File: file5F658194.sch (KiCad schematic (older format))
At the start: 21 parts, among them Q10 SUD50P10-43L, Q11 TIP120

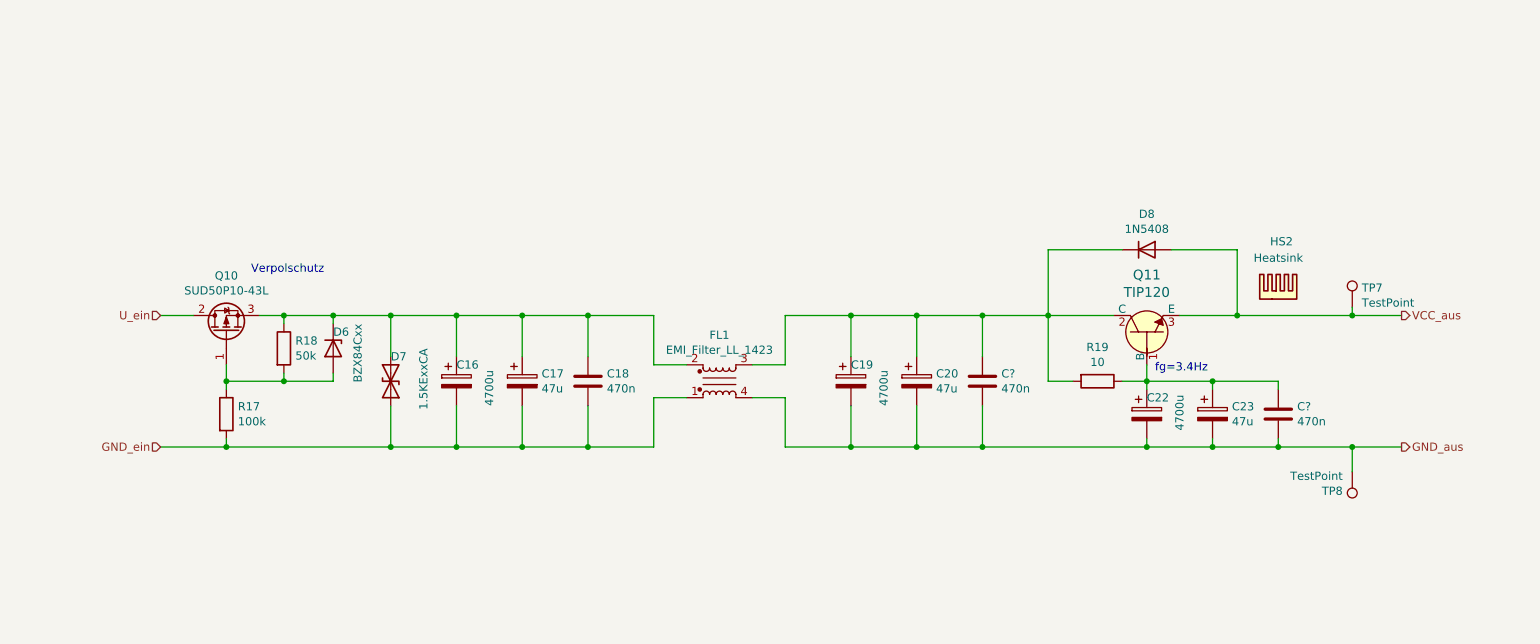
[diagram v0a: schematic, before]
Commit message: pcb netzteil rev. 1.0 finished
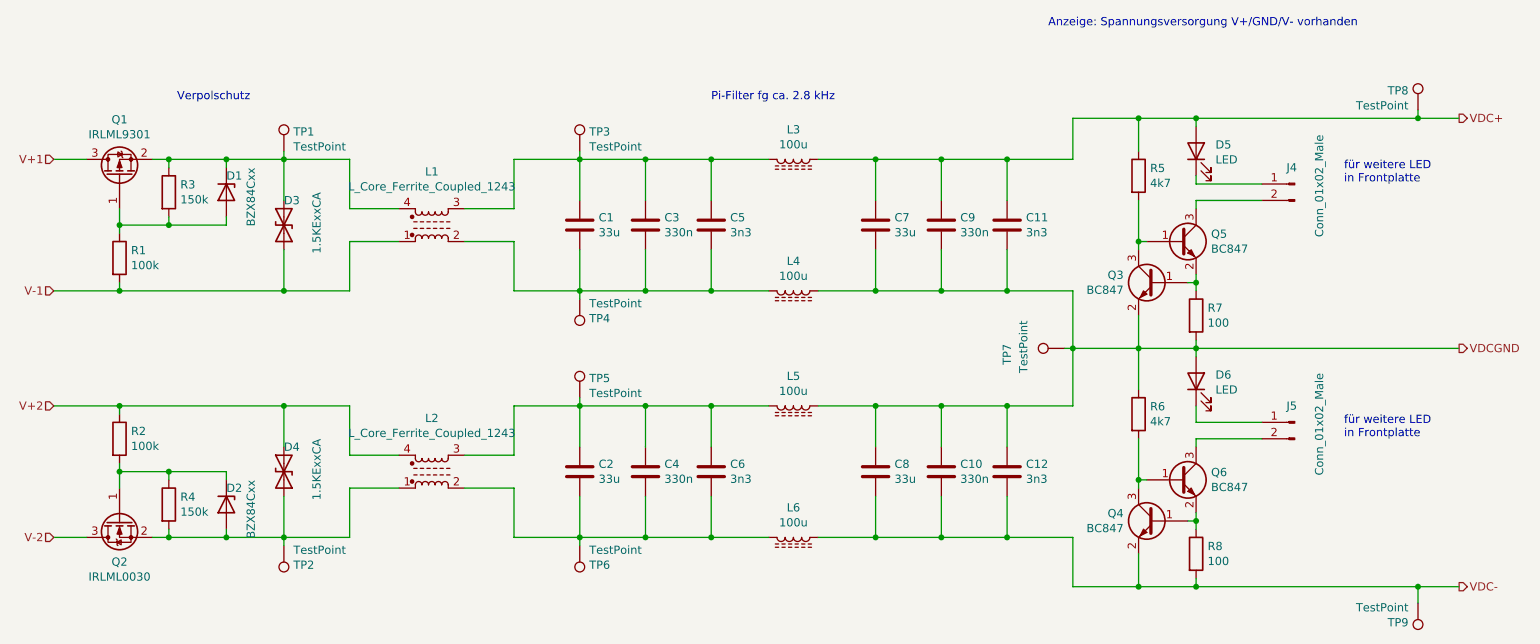
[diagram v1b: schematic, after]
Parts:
- removed C16, C19, C22: 4700u, Capacitor_THT:CP_Radial_D22.0mm_P10.00mm_SnapIn, symbol Device:CP
- removed C17, C23: 47u, Capacitor_THT:CP_Radial_D6.3mm_P2.50mm, symbol Device:CP
- removed C18, C? (x2): 470n, Capacitor_SMD:C_1206_3216Metric_Pad1.42x1.75mm_HandSolder, symbol Device:C
- removed C20: 47u, Capacitor_THT:CP_Radial_D5.0mm_P2.50mm, symbol Device:CP
- removed D8: 1N5408, Diode_THT:D_DO-201AD_P15.24mm_Horizontal, symbol Diode:1N5408
- removed FL1: EMI_Filter_LL_1423, symbol Device:EMI_Filter_LL_1423
- removed HS2: Heatsink, Heatsink:Heatsink_Fischer_SK129-STS_42x25mm_2xDrill2.5mm, symbol Mechanical:Heatsink
- removed Q10: SUD50P10-43L, Package_TO_SOT_SMD:TO-252-2, symbol Transistor_FET:SUD50P10-43L
- removed Q11: TIP120, digikey-footprints:TO-220-3, symbol dk_Transistors-Bipolar-BJT-Single:TIP120
- removed R19: 10, Resistor_SMD:R_1206_3216Metric_Pad1.42x1.75mm_HandSolder, symbol Device:R
- added C1, C2, C7, C8: 33u, Capacitor_SMD:C_1206_3216Metric_Pad1.42x1.75mm_HandSolder, symbol Device:C
- added C10, C3, C4, C9: 330n, Capacitor_SMD:C_1206_3216Metric_Pad1.42x1.75mm_HandSolder, symbol Device:C
- added C11, C12, C5, C6: 3n3, Capacitor_SMD:C_1206_3216Metric_Pad1.42x1.75mm_HandSolder, symbol Device:C
- added D2: BZX84Cxx, Diode_SMD:D_SOT-23_ANK, symbol Diode:BZX84Cxx
- added D4: 1.5KExxCA, Diode_THT:D_DO-201AE_P15.24mm_Horizontal, symbol Diode:1.5KExxCA
- added D5, D6: LED, LED_SMD:LED_1206_3216Metric_Pad1.42x1.75mm_HandSolder, symbol Device:LED
- added J4, J5: Conn_01x02_Male, Connector_PinHeader_2.54mm:PinHeader_1x02_P2.54mm_Vertical, symbol Connector:Conn_01x02_Male
- added L1, L2: L_Core_Ferrite_Coupled_1243, footprints:744822301, symbol Device:L_Core_Ferrite_Coupled_1243
- added L3, L4, L5, L6: 100u, Inductor_THT:L_Radial_D10.5mm_P5.00mm_Abacron_AISR-01, symbol Device:L_Core_Ferrite
- added Q1: IRLML9301, Package_TO_SOT_SMD:SOT-23, symbol Transistor_FET:IRLML9301
- added Q2: IRLML0030, Package_TO_SOT_SMD:SOT-23, symbol Transistor_FET:IRLML0030
- added Q3, Q4, Q5, Q6: BC847, Package_TO_SOT_SMD:SOT-23, symbol Transistor_BJT:BC847
- added R2: 100k, Resistor_SMD:R_1206_3216Metric_Pad1.42x1.75mm_HandSolder, symbol Device:R
- added R4: 150k, Resistor_SMD:R_1206_3216Metric_Pad1.42x1.75mm_HandSolder, symbol Device:R
- added R5, R6: 4k7, Resistor_SMD:R_1206_3216Metric_Pad1.42x1.75mm_HandSolder, symbol Device:R
- added R7, R8: 100, Resistor_SMD:R_1206_3216Metric_Pad1.42x1.75mm_HandSolder, symbol Device:R
- added TP2, TP3, TP4, TP5, TP6, TP8, TP9: TestPoint, TestPoint:TestPoint_Loop_D2.50mm_Drill1.0mm, symbol Connector:TestPoint
- R3: renamed from R18; value 50k -> 150k
- TP1: renamed from TP7; footprint TestPoint:TestPoint_Pad_D2.0mm -> TestPoint:TestPoint_Loop_D2.50mm_Drill1.0mm
- TP7: renamed from TP8; footprint TestPoint:TestPoint_Pad_D2.0mm -> TestPoint:TestPoint_Loop_D2.50mm_Drill1.0mm
- renumbered D6 to D1, D7 to D3, R17 to R1
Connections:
- net VCC_aus is gone; now on an unnamed net: TP1.1
- net at D1.1 (K), D3.1 (A1), R3.1: now also L1.4, Q1.2 (S)
- net at D1.2 (A), R1.1, R3.2: now also Q1.1 (G)
- net GND_aus renamed VDCGND
- net VDCGND: now also C10.1, C11.2, C12.1, C7.2, C8.1, C9.2, D6.2 (A), L4.1, L5.1, Q3.2 (E), R6.1, R7.2
- net GND_ein renamed V-1
- net V-1: now also L1.1
- new net: D2.2 (A), D4.2 (A2), L2.1, Q2.2 (S), R4.2, TP2.1
- new net: C1.1, C3.1, C5.1, L1.3, L3.2, TP3.1
- new net: C2.2, C4.2, C6.2, L2.2, L6.2, TP6.1
- new net: D2.1 (K), Q2.1 (G), R2.2, R4.1
- new net: C1.2, C3.2, C5.2, L1.2, L4.2, TP4.1
- new net: D6.1 (K), J5.1 (Pin_1)
- new net: Q4.3 (C), Q6.1 (B), R6.2
- new net: Q4.1 (B), Q6.2 (E), R8.1
- new net: J5.2 (Pin_2), Q6.3 (C)
- new net: C2.1, C4.1, C6.1, L2.3, L5.2, TP5.1
- new net: D5.1 (K), J4.1 (Pin_1)
- new net: Q3.3 (C), Q5.1 (B), R5.2
- new net: Q3.1 (B), Q5.2 (E), R7.1
- new net: J4.2 (Pin_2), Q5.3 (C)
- new net V+1: Q1.3 (D)
- new net V+2: D4.1 (A1), L2.4, R2.1
- new net V-2: Q2.3 (D)
- new net VDC+: C11.1, C7.1, C9.1, D5.2 (A), L3.1, R5.1, TP8.1
- new net VDC-: C10.2, C12.2, C8.2, L6.1, Q4.2 (E), R8.2, TP9.1
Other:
- note added: "Anzeige: Spannungsversorgung V+/GND/V- vorhanden"
- note added: "Pi-Filter fg ca. 2.8 kHz"
- note added: "für weitere LED \nin Frontplatte"
- note removed: "fg=3.4Hz"
- moved on the sheet: D1, D3, R1, R3, TP1, TP7
